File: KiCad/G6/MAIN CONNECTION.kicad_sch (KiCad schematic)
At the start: 19 parts, among them U10 TCA9543APWR, U8 IIM-42652 - Main Acceleromete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, U9 IIM-42652 Main Accelerometer

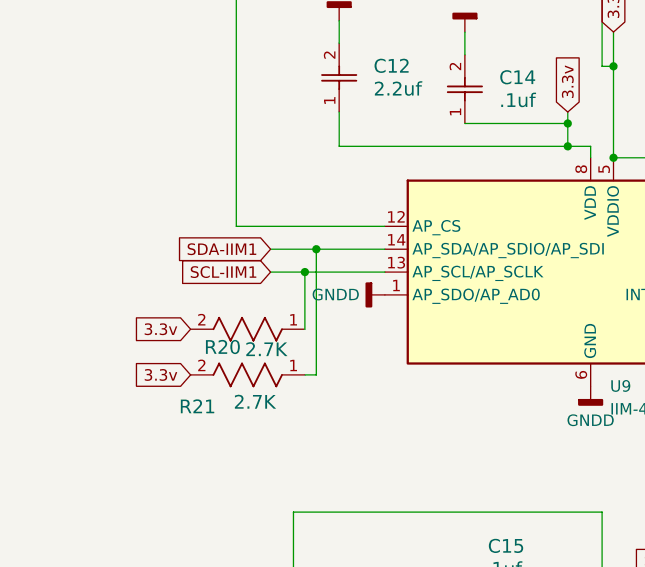
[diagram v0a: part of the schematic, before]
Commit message: i finally finished routing everything to spi
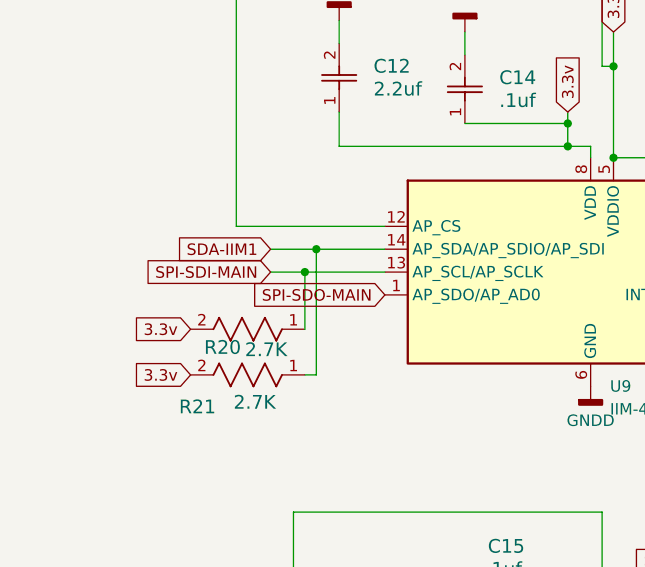
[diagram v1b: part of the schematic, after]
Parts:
- C12, C13: footprint CC0805KK7R7BB225:CAP_CC0805_YAG -> CC0603KRXQRQBB104:2.2CAP_CC1206_YAG
- C14, C15: footprint CC0603KRXQRQBB104:CC0603N_YAG -> CC0603KRXQRQBB104:.1CAP_CC1206_YAG
- C16, C17: footprint C0603C103K4RECTU:CAPC17595_87N_KEM -> CC0603KRXQRQBB104:.01YAG_CC1206_YAG
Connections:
- net GNDD: no longer U9.1 (AP_SDO/AP_AD0)
- net SCL-IIM1: no longer R20.1, U9.13 (AP_SCL/AP_SCLK)
- new net SPI-SDI-MAIN: R20.1, U9.13 (AP_SCL/AP_SCLK)
- new net SPI-SDO-MAIN: U9.1 (AP_SDO/AP_AD0)
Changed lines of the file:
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@@
+		)
+	)
+	(global_label "SPI-SDO-MAIN"
+		(shape input)
+		(at 73.66 73.66 180)
+		(fields_autoplaced yes)
+		(effects
+			(font
+				(size 1.27 1.27)
+			)
+			(justify right)
+		)
+		(property "Intersheetrefs" "${INTERSHEET_REFS}"
+			(at 56.1604 73.66 0)
+			(effects
+				(font
+					(size 1.27 1.27)
+				)
+				(justify right)
+				(hide yes)
+			)
 		)
 	)
@@
 		)
 	)
-	(global_label "SCL-IIM1"
+	(global_label "SPI-SDI-MAIN"
 		(shape input)
 		(at 60.96 71.12 180)
@@
 		)
 		(property "Intersheetrefs" "${INTERSHEET_REFS}"
-			(at 49.0243 71.12 0)
+			(at 44.1861 71.12 0)
 			(effects
 				(font
@@
 			)
 		)
-		(property "Footprint" "CC0603KRXQRQBB104:CC0603N_YAG"
+		(property "Footprint" "CC0603KRXQRQBB104:.1CAP_CC1206_YAG"
 			(at 91.44 107.95 0)
 			(effects
@@
 	)
 	(symbol
-		(lib_id "power:GNDD")
-		(at 73.66 73.66 270)
-		(unit 1)
-		(exclude_from_sim no)
-		(in_bom yes)
-		(on_board yes)
-		(dnp no)
-		(property "Reference" "#PWR035"
-			(at 67.31 73.66 0)
-			(effects
-				(font
-					(size 1.27 1.27)
-				)
-				(hide yes)
-			)
-		)
-		(property "Value" "GNDD"
-			(at 70.866 73.66 90)
-			(effects
-				(font
-					(size 1.27 1.27)
-				)
-				(justify right)
-			)
-		)
-		(property "Footprint" ""
-			(at 73.66 73.66 0)
-			(effects
-				(font
-					(size 1.27 1.27)
-				)
-				(hide yes)
-			)
-		)
-		(property "Datasheet" ""
-			(at 73.66 73.66 0)
-			(effects
-				(font
-					(size 1.27 1.27)
-				)
-				(hide yes)
-			)
-		)
-		(property "Description" "Power symbol creates a global label with name \"GNDD\" , digital ground"
-			(at 73.66 73.66 0)
-			(effects
-				(font
-					(size 1.27 1.27)
-				)
-				(hide yes)
-			)
-		)
-		(pin "1"
-		)
-		(instances
-			(project "G6"
-				(path "/99017594-210d-4d15-87a7-3152ef0d7b7c/1d29283e-2ace-44ea-9175-ec7a0e5b2450"
-					(reference "#PWR035")
-					(unit 1)
-				)
-			)
-		)
-	)
-	(symbol
 		(lib_id "2025-10-06_20-52-39:CRG0805F2K7")
 		(at 52.07 82.55 0)
@@
 			)
 		)
-		(property "Footprint" "CC0603KRXQRQBB104:CC0603N_YAG"
+		(property "Footprint" "CC0603KRXQRQBB104:.1CAP_CC1206_YAG"
 			(at 82.55 54.61 0)
 			(effects
@@
 			)
 		)
-		(property "Footprint" "C0603C103K4RECTU:CAPC17595_87N_KEM"
+		(property "Footprint" "CC0603KRXQRQBB104:.01YAG_CC1206_YAG"
 			(at 119.38 111.76 0)
 			(effects
@@
 			)
 		)
-		(property "Footprint" "CC0805KK7R7BB225:CAP_CC0805_YAG"
+		(property "Footprint" "CC0603KRXQRQBB104:2.2CAP_CC1206_YAG"
 			(at 87.63 119.38 0)
 			(effects
@@
 			)
 		)
-		(property "Footprint" "CC0805KK7R7BB225:CAP_CC0805_YAG"
+		(property "Footprint" "CC0603KRXQRQBB104:2.2CAP_CC1206_YAG"
 			(at 68.58 53.34 0)
 			(effects
@@
 			)
 		)
-		(property "Footprint" "C0603C103K4RECTU:CAPC17595_87N_KEM"
+		(property "Footprint" "CC0603KRXQRQBB104:.01YAG_CC1206_YAG"
 			(at 107.95 58.42 0)
 			(effects
